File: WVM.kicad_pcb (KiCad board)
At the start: 2 copper layers, 23.3 x 27.6 mm, 35 parts, among them J1 USB4215-03-A_REVA, J2 Conn_01x02_Pin, Q1 BSS138, Q2 BSS138, SW1 SW_SPST, SW2 SW_SPST, U1 NORA-W106-00B, U2 CH340C, U3 IIS3DWBTR, U4 TPS63036YFGT, U5 TP4056-42-ESOP8, U6 MCP9808_DFN

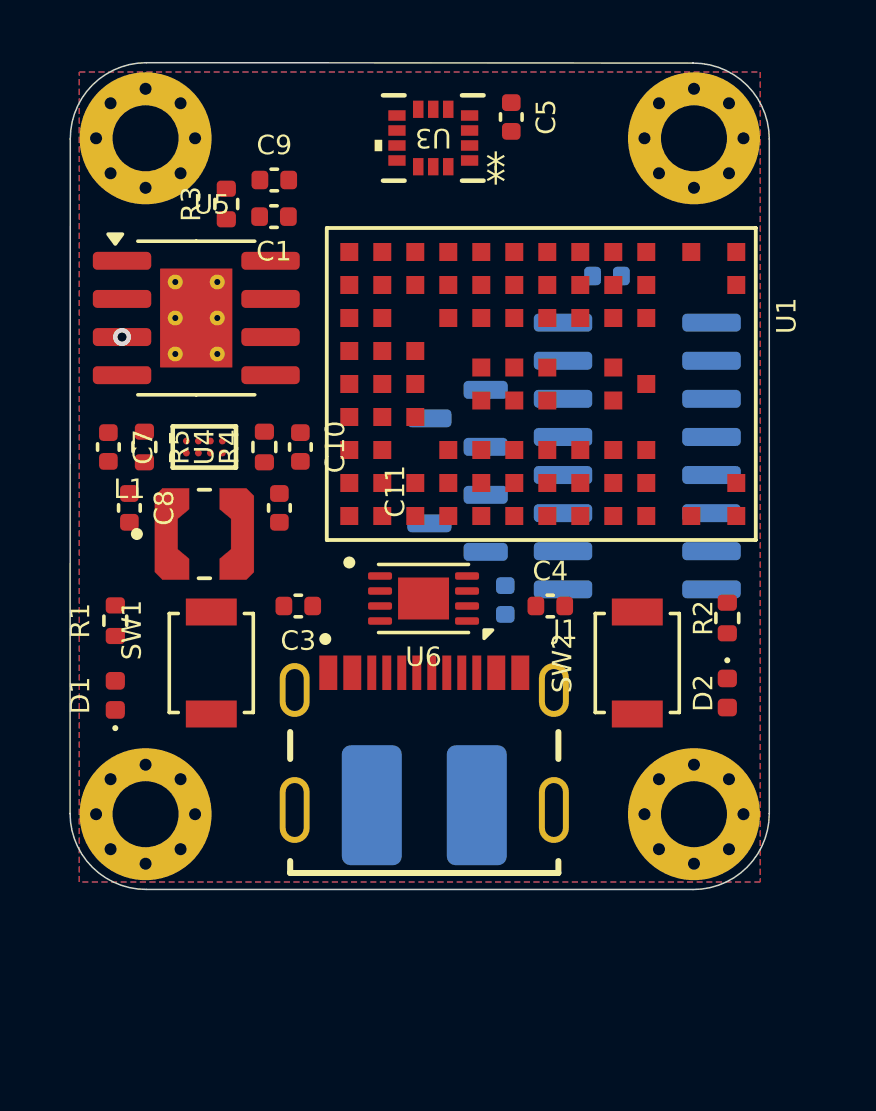
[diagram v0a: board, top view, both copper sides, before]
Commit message: 17102025
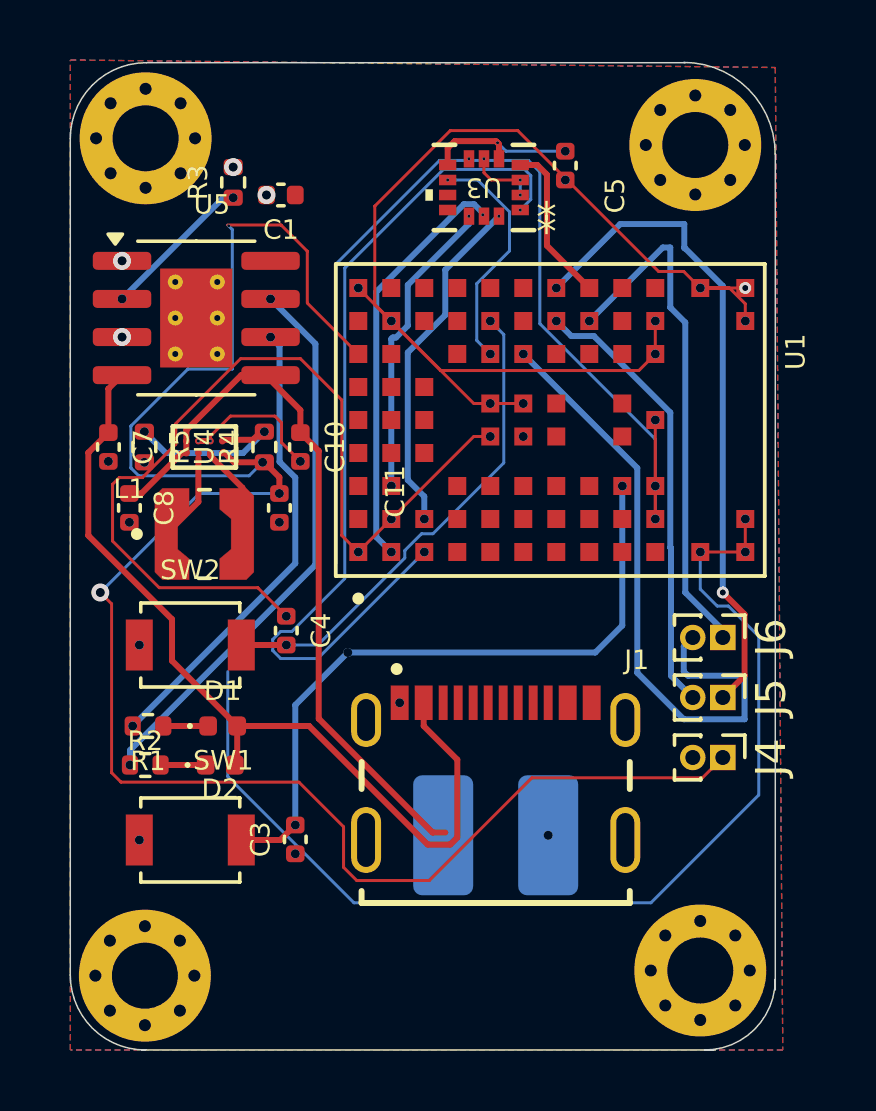
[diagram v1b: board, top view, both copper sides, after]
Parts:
- removed C2, C9: 0.1uF, Capacitor_SMD:C_0402_1005Metric
- removed C6: 1uF, Capacitor_SMD:C_0402_1005Metric
- removed Q1, Q2: BSS138, Package_TO_SOT_SMD:SOT-23
- removed U2: CH340C, Package_SO:SOIC-16_3.9x9.9mm_P1.27mm
- removed U6: MCP9808_DFN, Package_DFN_QFN:DFN-8-1EP_3x2mm_P0.5mm_EP1.7x1.4mm
- added J4: Conn_01x02_Pin, Connector_PinHeader_1.00mm:PinHeader_1x02_P1.00mm_Vertical, F.Cu at (237.8, 131.8)
- added J5: Conn_01x02_Pin, Connector_PinHeader_1.00mm:PinHeader_1x02_P1.00mm_Vertical, F.Cu at (237.8, 129.8)
- added J6: Conn_01x02_Pin, Connector_PinHeader_1.00mm:PinHeader_1x02_P1.00mm_Vertical, F.Cu at (237.8, 127.8)
- moved R2 20.0 mm to (218.5, 132.0), turned to 180 degrees
- moved D2 17.1 mm to (221.0, 132.0), turned to 0 degrees
- moved SW2 14.9 mm to (220.0, 128.0), turned to 0 degrees
- moved C4 8.84 mm to (223.2, 127.5), turned to -90 degrees
- moved C3 7.78 mm to (223.5, 134.5), turned to 90 degrees
- moved SW1 5.94 mm to (220.0, 134.5), turned to 0 degrees
- moved H4 5.38 mm to (218.5, 139.0)
- moved H1 5.21 mm to (237.0, 138.8)
- moved D1 3.72 mm to (221.1, 130.7), turned to 0 degrees
- moved R1 3.68 mm to (218.6, 130.7), turned to 180 degrees
- moved J1 2.58 mm to (230.2, 134.5)
- moved J2 2.58 mm to (230.2, 131.8)
- moved C5 2.42 mm to (232.5, 112.0)
- moved U3 2.36 mm to (229.8, 112.7)
- moved U1 1.24 mm to (232.0, 120.5)
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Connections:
- J1 pad A6: D+ -> unconnected-(J1-DP1-PadA6)
- J1 pad A7: D- -> unconnected-(J1-DN1-PadA7)
- J2 pad 2: -BAT -> GND
- U1 pad A2: SCL -> unconnected-(U1-FSPIWP/GPIO38-PadA2)
- U1 pad D3: SDA -> unconnected-(U1-FSPIHD/GPIO33-PadD3)
- U1 pad E7: unconnected-(U1-GPIO9-PadE7) -> INT2
- U1 pad H8: unconnected-(U1-GPIO2-PadH8) -> EN
- U1 pad H9: unconnected-(U1-GPIO8-PadH9) -> INT1
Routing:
- net GND: track 0.00 -> 148.3 mm, vias 1 -> 43
- net 3V3: track 0.00 -> 68.1 mm, vias 0 -> 7
- net Net-(D1-A): track 0.00 -> 29.6 mm
- net MISO: track 0.00 -> 29.5 mm, vias 0 -> 2
- net +BAT: track 0.00 -> 24.7 mm
- net RESET: track 0.00 -> 22.7 mm, vias 0 -> 3
- net RX: track 0.00 -> 22.1 mm, vias 0 -> 3
- net BOOT: track 0.00 -> 21.2 mm, vias 0 -> 2
- net Net-(U5-~{CHRG}): track 0.00 -> 18.7 mm, vias 0 -> 2
- net EN: track 0.00 -> 17.4 mm, vias 0 -> 2
- net GPIO1: track 0.00 -> 16.3 mm, vias 0 -> 2
- net Net-(U5-~{STDBY}): track 0.00 -> 15.6 mm, vias 0 -> 2
- net TX: track 0.00 -> 14.9 mm, vias 0 -> 2
- net CLK: track 0.00 -> 13.8 mm, vias 0 -> 2
- net MOSI: track 0.00 -> 11.8 mm, vias 0 -> 2
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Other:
- board size 23.3 x 27.6 mm -> 23.5 x 32.9 mm
